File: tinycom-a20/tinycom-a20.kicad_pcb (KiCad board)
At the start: 4 copper layers, 40.4 x 41.9 mm, 35 parts, among them P1 CONN_02X10, P2 CONN_02X10, P3 CONN_01X01, U1 ALLWINNERA10/TFBGA441, U2 H5TQG63BFR/FBGA96, Y1 Crystal_Small, Y2 Crystal_Small

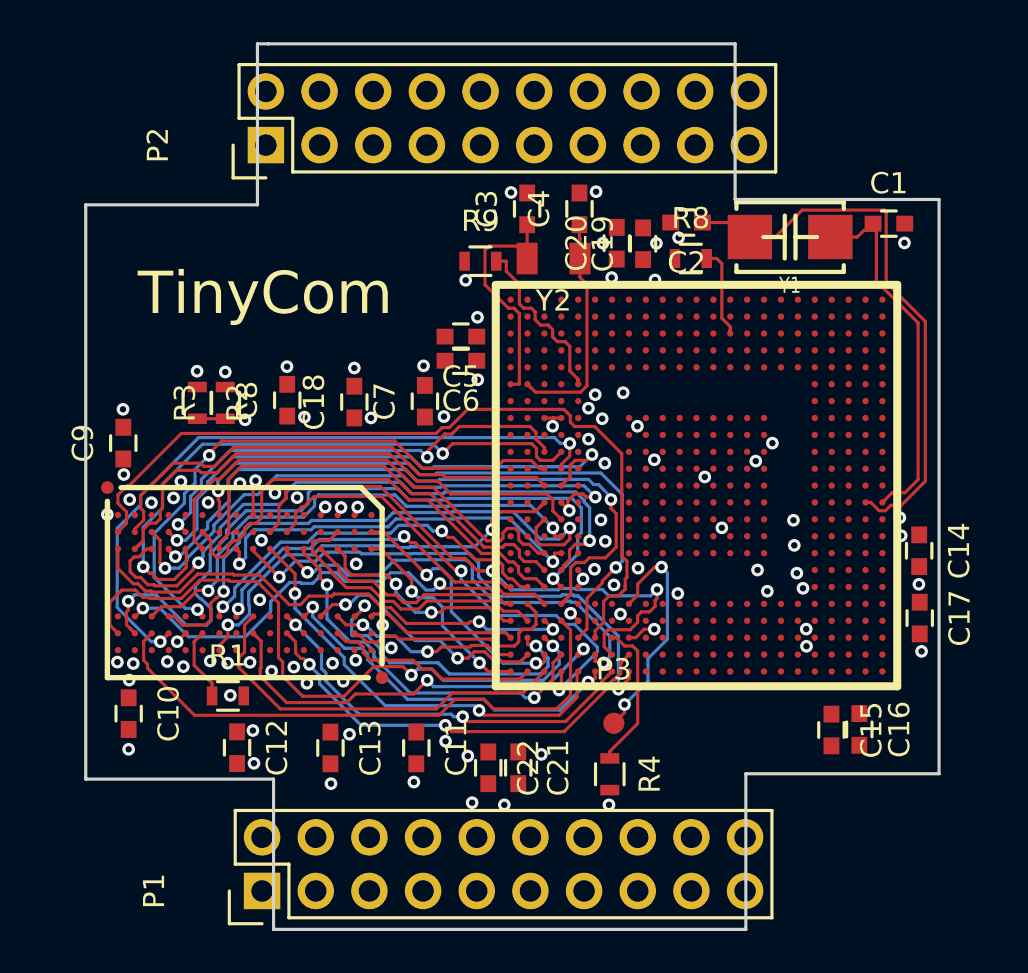
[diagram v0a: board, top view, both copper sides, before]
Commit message: improve placement
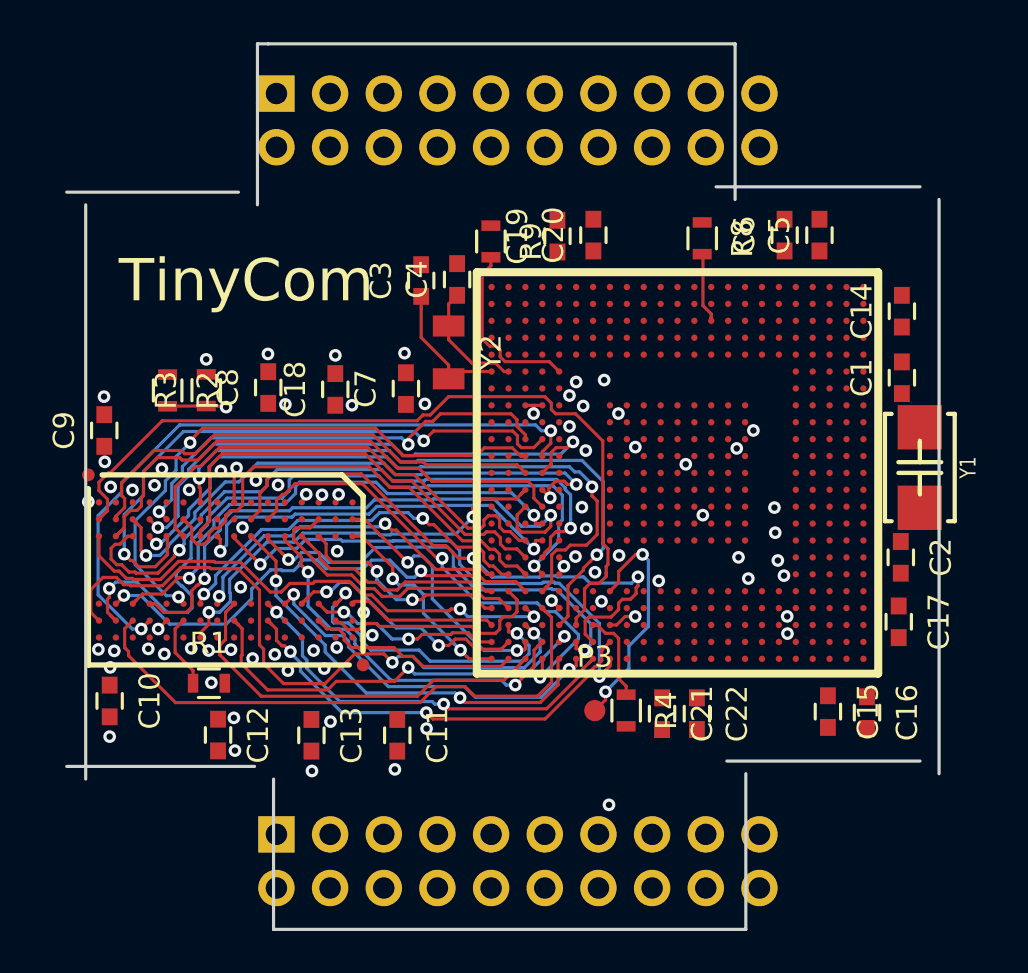
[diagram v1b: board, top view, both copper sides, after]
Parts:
- P1, P2: moved to B.Cu
- R1, R4: value R_Small -> 330R
- R2, R3: value R_Small -> 2K
- moved C2 18.8 mm to (123.4, 144.4), turned to 270 degrees
- moved C5 17.6 mm to (119.6, 129.2), turned to 90 degrees
- moved C6 16.4 mm to (117.9, 129.2), turned to 90 degrees
- moved Y1 12.5 mm to (124.3, 140.2), turned to 90 degrees
- moved C14 11.4 mm to (123.5, 132.8), turned to 90 degrees
- moved C22 10.2 mm to (113.8, 151.8)
- moved C1 7.32 mm to (123.5, 135.9), turned to 90 degrees
- moved C21 7.27 mm to (112.1, 151.8)
- moved C4 6.69 mm to (102.4, 131.3)
- moved C3 6.06 mm to (100.7, 131.3)
- moved C19 4.07 mm to (107.2, 129.2)
- moved Y2 3.14 mm to (104.5, 134.7), turned to 270 degrees
- moved R4 3.11 mm to (110.4, 151.7)
- moved P1 2.76 mm to (93.9, 157.6), turned to 270 degrees
- moved P2 2.49 mm to (93.9, 122.5), turned to 270 degrees
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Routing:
- net Net-(C2-Pad1): track 26.6 -> 0.00 mm
- net Net-(C1-Pad1): track 17.7 -> 0.00 mm
- net Net-(C4-Pad1): track 11.1 -> 5.72 mm
- net Net-(C3-Pad1): track 11.3 -> 6.61 mm
- net Net-(R4-Pad1): track 7.10 -> 4.29 mm
- net RESET#: track 4.45 -> 3.50 mm
- net SVREF: track 48.8 -> 49.3 mm
- net (no net): vias 97 -> 77
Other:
- board size 40.4 x 41.9 mm -> 41.3 x 41.9 mm
